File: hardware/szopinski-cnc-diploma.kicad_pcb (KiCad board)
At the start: 4 copper layers, 99.1 x 58.4 mm, 29 parts, among them J1 Barrel_Jack, J2 Conn_02x08_Odd_Even, J3 AVR-ISP-10, J4 Conn_01x04, J5 Conn_01x04, J6 Conn_01x04, J7 Conn_01x04, U1 ATmega328P-PU, U2 L7805, U3 DRV8825, U4 DRV8825, U5 DRV8825, U6 DRV8825, Y1 20 MHz

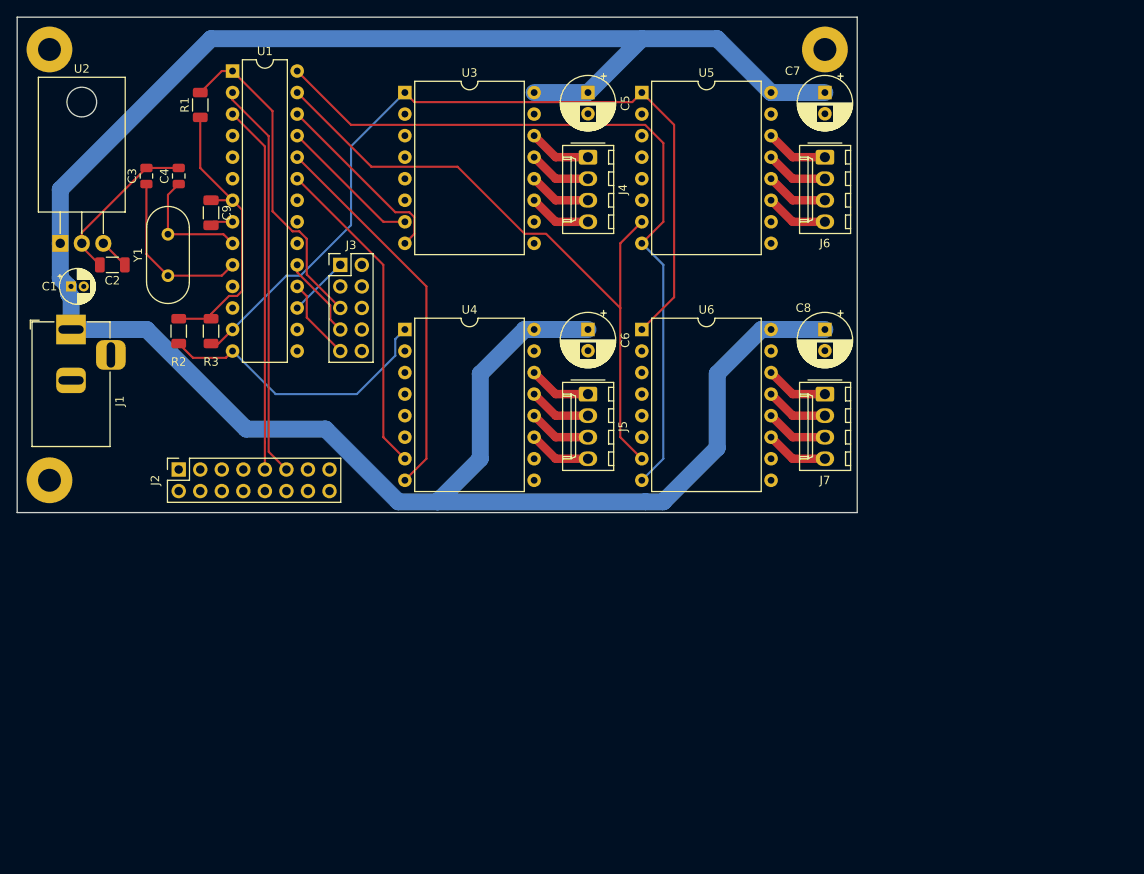
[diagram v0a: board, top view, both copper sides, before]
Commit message: Redesign PCB
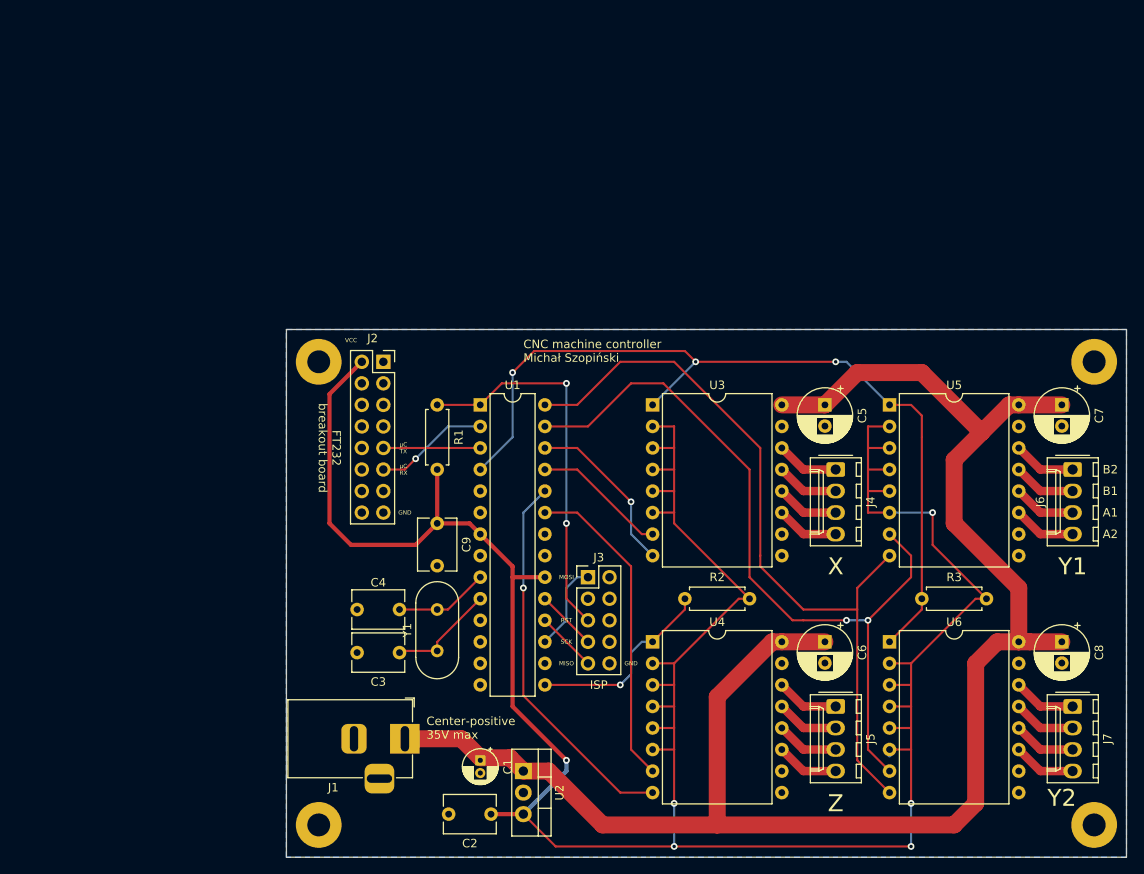
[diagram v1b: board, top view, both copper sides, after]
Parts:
- removed the REF** at (77.5, 47.0)
- removed the REF** at (168.9, 47.0)
- removed the REF** at (77.5, 97.8)
- added REF**: MountingHole_2.7mm_Pad, MountingHole:MountingHole_2.7mm_Pad, F.Cu at (109.2, 138.4)
- added REF**: MountingHole_2.7mm_Pad, MountingHole:MountingHole_2.7mm_Pad, F.Cu at (200.7, 138.4)
- added REF**: MountingHole_2.7mm_Pad, MountingHole:MountingHole_2.7mm_Pad, F.Cu at (200.7, 83.8)
- added REF**: MountingHole_2.7mm_Pad, MountingHole:MountingHole_2.7mm_Pad, F.Cu at (109.2, 83.8)
- C2, C9: footprint Capacitor_SMD:C_1206_3216Metric -> Capacitor_THT:C_Disc_D6.0mm_W4.4mm_P5.00mm
- C3, C4: footprint Capacitor_SMD:C_0805_2012Metric -> Capacitor_THT:C_Disc_D6.0mm_W4.4mm_P5.00mm
- C5, C6, C7, C8: value CP -> 100u
- R1, R2, R3: footprint Resistor_SMD:R_1206_3216Metric -> Resistor_THT:R_Axial_DIN0207_L6.3mm_D2.5mm_P7.62mm_Horizontal
- U2: footprint Package_TO_SOT_THT:TO-220-3_Horizontal_TabDown -> Package_TO_SOT_THT:TO-220-3_Vertical
- moved R3 96.7 mm to (188.0, 111.8), turned to 180 degrees
- moved U2 82.8 mm to (133.3, 132.1), turned to 270 degrees
- moved C2 78.7 mm to (129.5, 137.2)
- moved R2 74.3 mm to (160.0, 111.8), turned to 180 degrees
- moved C1 73.8 mm to (128.3, 130.8), turned to 270 degrees
- moved C3 63.6 mm to (118.7, 118.1), turned to 180 degrees
- moved J1 62.3 mm to (119.4, 128.3), turned to 0 degrees
- moved C4 57.4 mm to (118.7, 113.0), turned to 180 degrees
- moved Y1 54.5 mm to (123.2, 117.9)
- moved R1 51.3 mm to (123.2, 96.5)
- moved U1 49.0 mm to (128.3, 88.9)
- moved J4 47.0 mm to (170.2, 96.5)
- moved J5 47.0 mm to (170.2, 124.5)
- moved J6 47.0 mm to (198.1, 96.5)
- moved J7 47.0 mm to (198.1, 124.5)
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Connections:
- U1 pad 13: /ENABLE_XY -> Net-(U1-Pad13)
- U1 pad 14: /ENABLE_Z -> Net-(U1-Pad14)
- U1 pad 15: Net-(U1-Pad15) -> /ENABLE_Z
- U1 pad 4: Net-(U1-Pad4) -> /ENABLE_XY
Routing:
- net +5V: track 37.8 -> 312.5 mm, vias 0 -> 6
- net +18V: track 276.3 -> 198.8 mm
- net /RXD: track 47.1 -> 13.5 mm, vias 0 -> 1
- net /TXD: track 43.5 -> 11.4 mm
- net GND: track 22.0 -> 0.00 mm
- net /STEP_Y: track 78.7 -> 91.4 mm, vias 0 -> 2
- net /ENABLE_Z: track 34.1 -> 23.0 mm, vias 0 -> 1
- net Net-(C3-Pad1): track 20.5 -> 13.4 mm
- net /RESET: track 38.5 -> 45.3 mm, vias 0 -> 2
- net Net-(J3-Pad1): track 7.18 -> 10.5 mm
- net Net-(C4-Pad1): track 15.0 -> 11.7 mm
- net Net-(J3-Pad7): track 9.72 -> 7.18 mm
- net Net-(J3-Pad9): track 9.72 -> 7.18 mm
- net /DIR_X: track 22.4 -> 20.2 mm, vias 0 -> 1
- net /STEP_X: track 16.9 -> 15.9 mm
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- added copper zone on B.Cu, net GND
- removed copper zone on In1.Cu, net +5V
- removed copper zone on In2.Cu, net GND
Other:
- board size 99.1 x 58.4 mm -> 99.1 x 62.2 mm
- copper layers 4 -> 2
- board text added: "A1"
- board text added: "A2"
- board text added: "B1"
- board text added: "B2"
- board text added: "CNC machine controller Michał Szopiński"
- board text added: "Center-positive 35V max"
- board text added: "FT232 breakout board"
- board text added: "GND"
- board text added: "ISP"
- board text added: "MISO"
- board text added: "MOSI"
- board text added: "RST"
- board text added: "SCK"
- board text added: "VCC"
- board text added: "X"
- board text added: "Y1"
- board text added: "Y2"
- board text added: "Z"
- board text added: "μC RX"
- board text added: "μC TX"
